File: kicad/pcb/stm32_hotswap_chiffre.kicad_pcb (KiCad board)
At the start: 2 copper layers, 227.3 x 85 mm, 109 parts, among them J1 USB_C_Receptacle_USB2.0, J101 Conn_01x03_Female, J2 OLED I2C, SW1 SW_Push, SW10 SW_Push, SW11 SW_Push, SW12 SW_Push, SW13 SW_Push, SW14 SW_Push, SW15 SW_Push, SW16 SW_Push, SW17 SW_Push, SW18 SW_Push, SW19 SW_Push, SW2 SW_Push, SW20 SW_Push, SW21 SW_Push, SW22 SW_Push, SW23 SW_Push, SW24 SW_Push, SW25 SW_Push, SW26 SW_Push, SW27 SW_Push, SW28 SW_Push, SW29 SW_Push, SW3 SW_Push, SW30 SW_Push, SW31 SW_Push, SW32 SW_Push, SW33 SW_Push, SW34 SW_Push, SW35 SW_Push, SW36 Rotary_Encoder_Switch, SW37 SKQGABE010, SW4 SW_Push, SW5 SW_Push, SW6 SW_Push, SW7 SW_Push, SW8 SW_Push, SW9 SW_Push, U1 STM32F072CBT6, U2 PRTR5V0U2X, U3 XC6206PxxxMR-Regulator_Linear

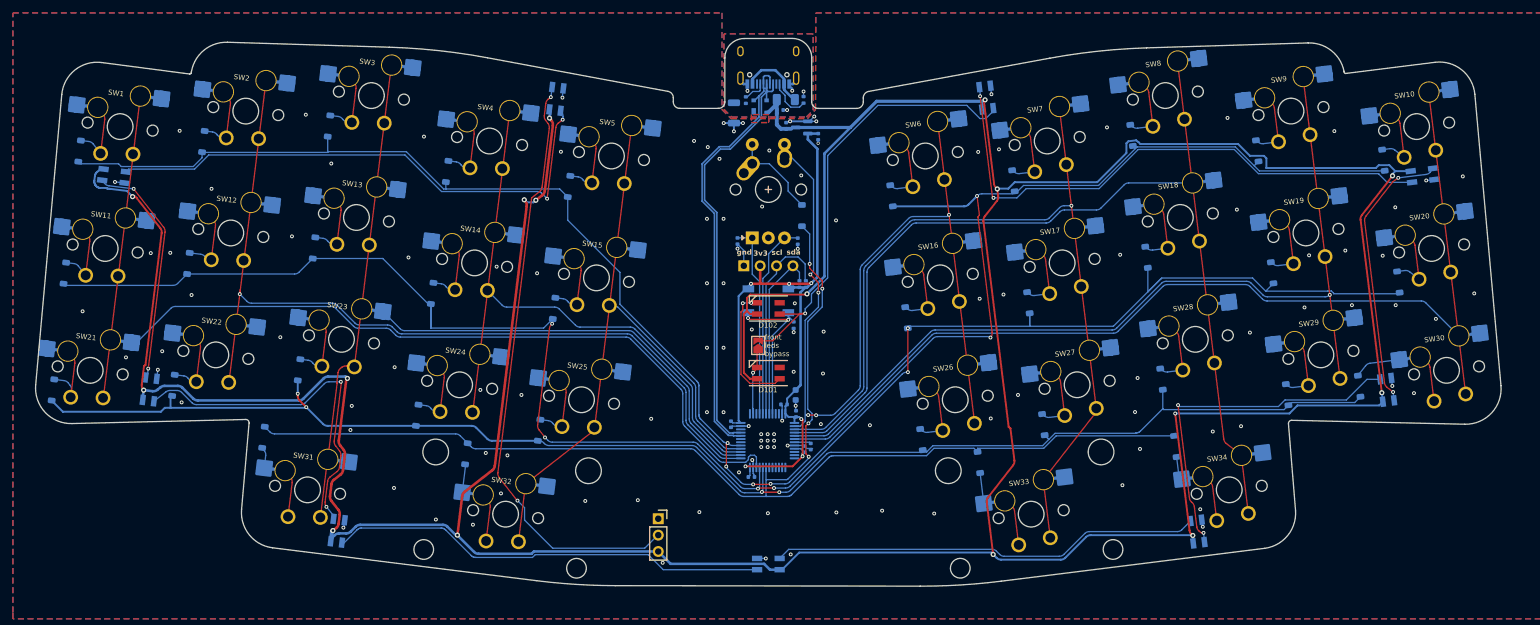
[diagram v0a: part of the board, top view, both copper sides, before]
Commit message: v0.2.2
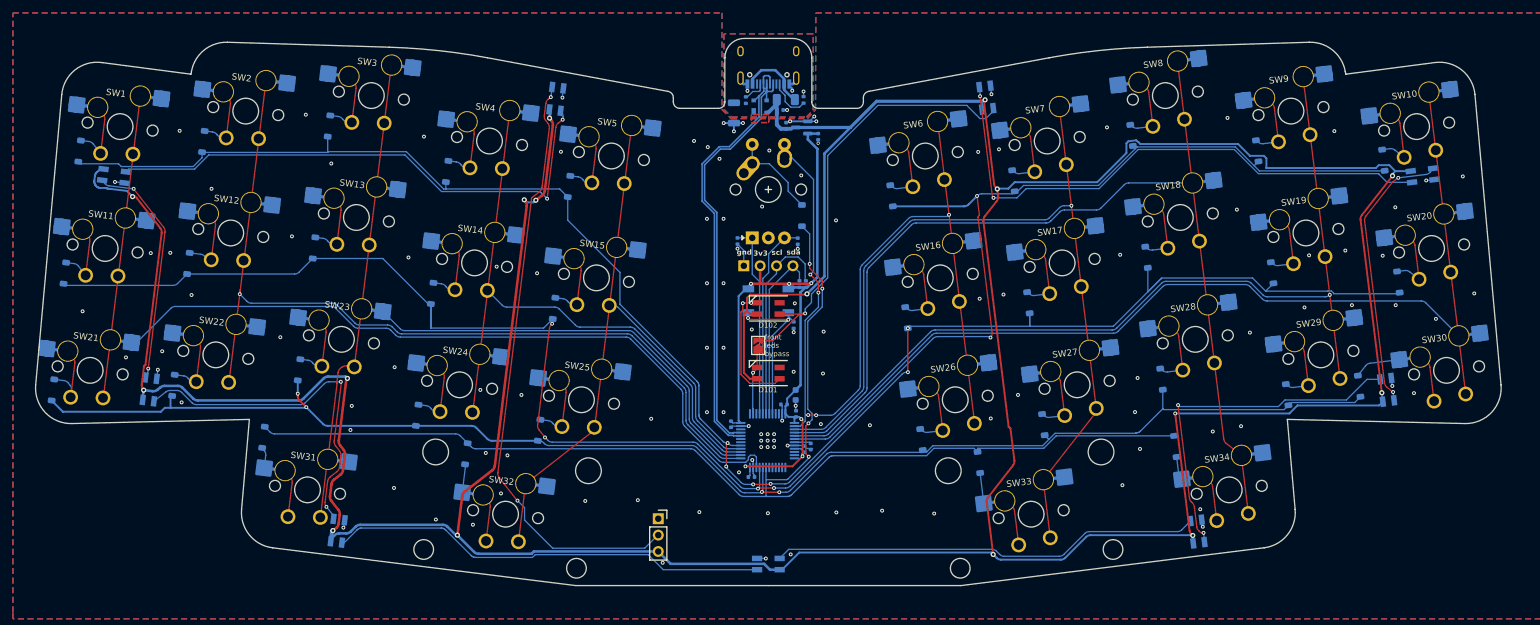
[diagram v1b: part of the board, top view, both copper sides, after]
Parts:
- SW36: footprint modified_footrprints:RotaryEncoder_EC11_no_mp -> modified_footprints:RotaryEncoder_EC11_no_mp
- SW37: footprint modified_footrprints:SW_SPST_SKQG_WithoutStem -> modified_footprints:SW_SPST_SKQG_WithoutStem
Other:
- board size 227.3 x 85 mm -> 227.4 x 84.9 mm
